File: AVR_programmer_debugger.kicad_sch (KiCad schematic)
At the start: 21 parts, among them J1 Flipper Zero, J2 AVR-UPDI-6, J3 Conn_01x04, J4 AVR-ISP-10, SW1 SW_SPDT, U1 TXS0104EPWR, U2 TXS0104EPWR

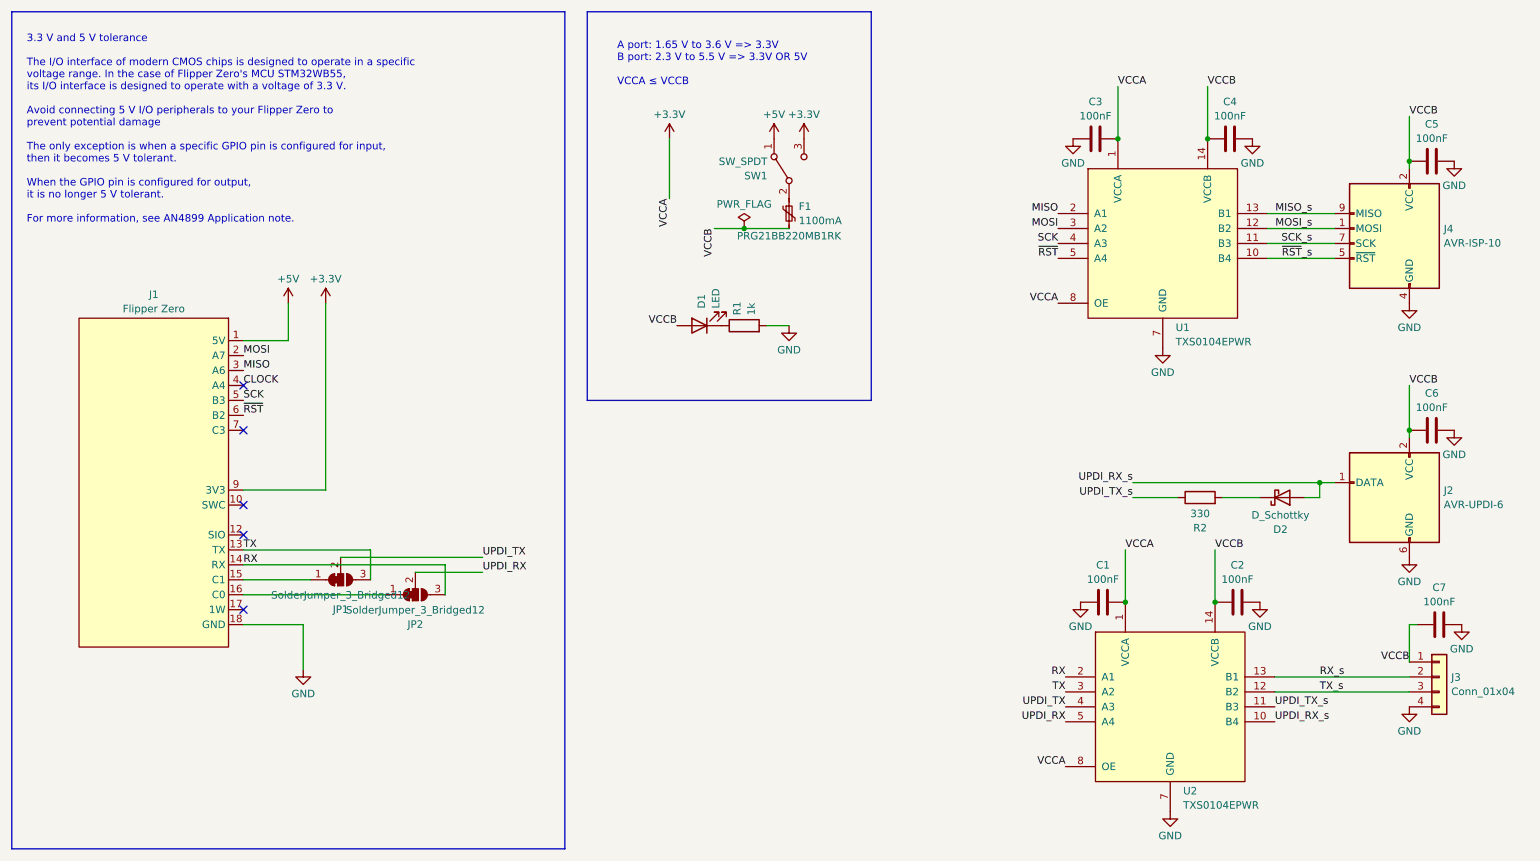
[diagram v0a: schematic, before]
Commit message: V1.2
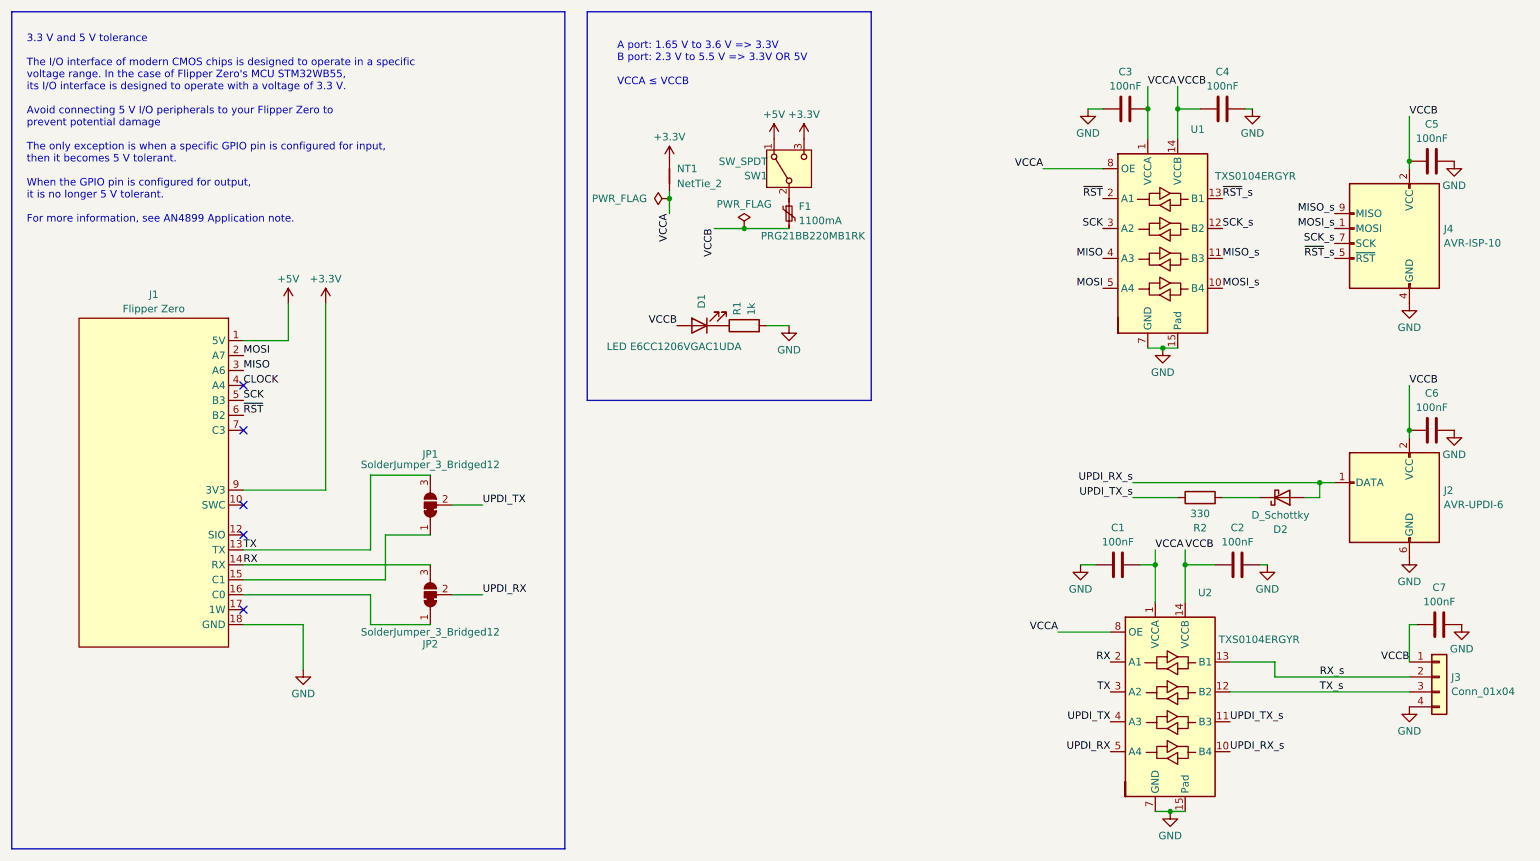
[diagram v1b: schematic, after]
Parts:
- added NT1: NetTie_2, NetTie:NetTie-2_SMD_Pad0.5mm, symbol Device:NetTie_2
- D1: value LED -> LED E6CC1206VGAC1UDA; Field4 (none) -> E6CC1206VGAC1UDA
- JP1, JP2: now left out of the parts list
- U1, U2: value TXS0104EPWR -> TXS0104ERGYR; footprint Package_SO:TSSOP-14_4.4x5mm_P0.65mm -> Package_DFN_QFN:Texas_S-PVQFN-N14_ThermalVias; symbol AlfaProxima:TXS0104EPWR-Logic_LevelTranslator -> Logic_LevelTranslator:TXB0104RGY
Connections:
- net +3.3V: now also NT1.1; no longer C1.2, C3.2, U1.1 (VCCA), U1.8 (OE), U2.1 (VCCA), U2.8 (OE)
- net GND: now also U1.15 (Pad), U2.15 (Pad)
- net MISO: now also U1.4 (A3); no longer U1.2 (A1)
- net MISO_s: now also U1.11 (B3); no longer U1.13 (B1)
- net MOSI: now also U1.5 (A4); no longer U1.3 (A2)
- net MOSI_s: now also U1.10 (B4); no longer U1.12 (B2)
- net SCK: now also U1.3 (A2); no longer U1.4 (A3)
- net SCK_s: now also U1.12 (B2); no longer U1.11 (B3)
- net ~{RST}: now also U1.2 (A1); no longer U1.5 (A4)
- net ~{RST}_s: now also U1.13 (B1); no longer U1.10 (B4)
- new net VCCA: C1.2, C3.2, NT1.2, U1.1 (VCCA), U1.8 (OE), U2.1 (VCCA), U2.8 (OE)
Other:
- moved on the sheet: C1, C2, C3, C4, JP1, JP2
